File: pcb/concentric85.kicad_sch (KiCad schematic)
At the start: 176 parts, among them J1 USB_C_Receptacle_USB2.0, SW1 SW_Push, SW10 SW_Push, SW11 SW_Push, SW12 SW_Push, SW13 SW_Push, SW14 SW_Push, SW15 SW_Push, SW16 SW_Push, SW17 SW_Push, SW18 SW_Push, SW19 SW_Push, SW2 SW_Push, SW20 SW_Push, SW21 SW_Push, SW22 SW_Push, SW23 SW_Push, SW24 SW_Push, SW25 SW_Push, SW26 SW_Push, SW27 SW_Push, SW28 SW_Push, SW29 SW_Push, SW3 SW_Push, SW30 SW_Push, SW31 SW_Push, SW32 SW_Push, SW33 SW_Push, SW34 SW_Push, SW35 SW_Push, SW36 SW_Push, SW37 SW_Push, SW38 SW_Push, SW39 SW_Push, SW4 SW_Push, SW40 SW_Push, SW41 SW_Push, SW42 SW_Push, SW43 SW_Push, SW44 SW_Push, SW45 SW_Push, SW46 SW_Push, SW47 SW_Push, SW48 SW_Push, SW49 SW_Push, SW5 SW_Push, SW50 SW_Push, SW51 SW_Push, SW52 SW_Push, SW53 SW_Push, SW54 SW_Push, SW55 SW_Push, SW56 SW_Push, SW57 SW_Push, SW58 SW_Push, SW59 SW_Push, SW6 SW_Push, SW60 SW_Push, SW61 SW_Push, SW62 SW_Push, SW63 SW_Push, SW64 SW_Push, SW65 SW_Push, SW66 SW_Push, SW67 SW_Push, SW68 SW_Push, SW69 SW_Push, SW7 SW_Push, SW70 SW_Push, SW71 SW_Push, SW72 SW_Push, SW73 SW_Push, SW74 SW_Push, SW75 SW_Push, SW76 SW_Push, SW77 SW_Push, SW78 SW_Push, SW79 SW_Push, SW8 SW_Push, SW80 SW_Push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

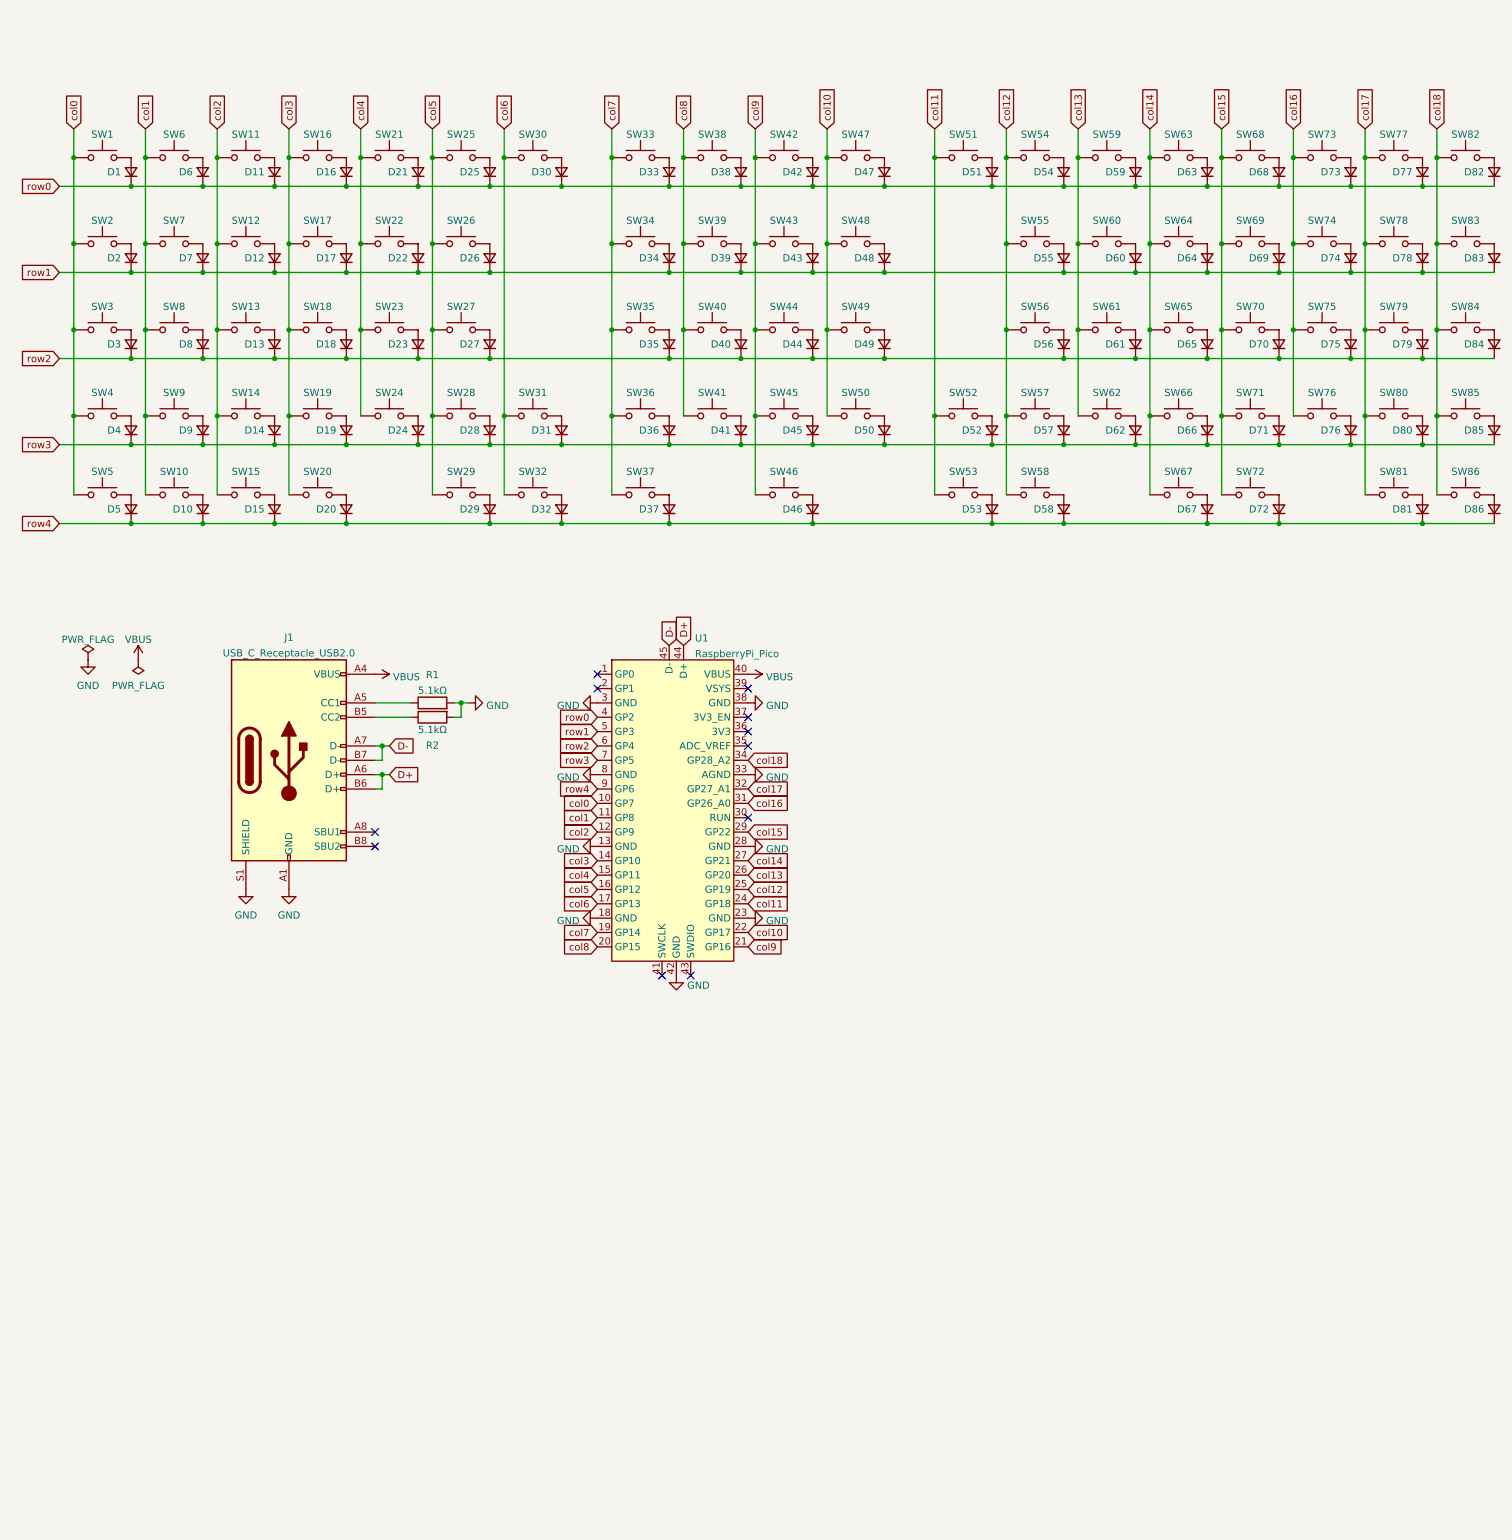
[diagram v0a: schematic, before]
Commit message: backup
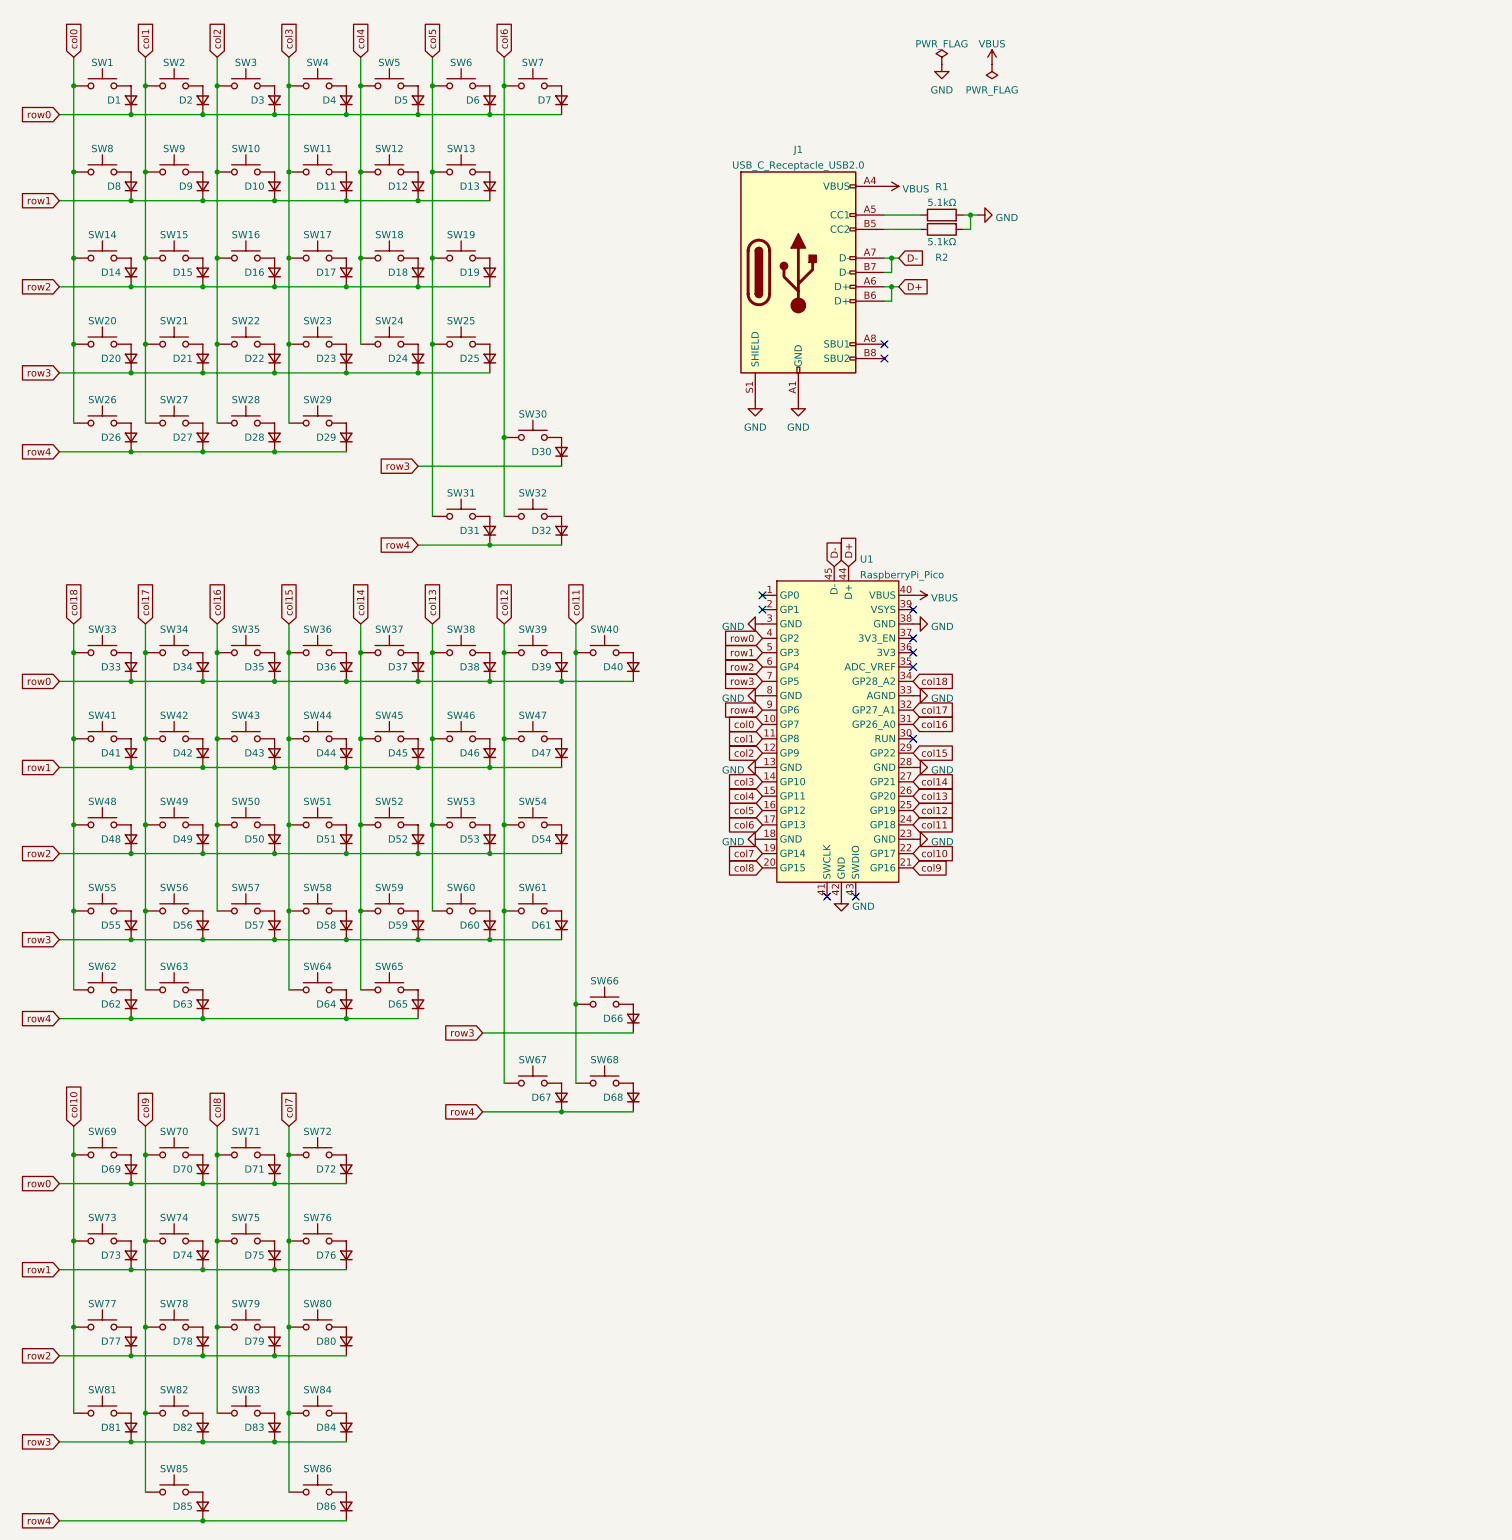
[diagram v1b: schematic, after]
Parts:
- R1, R2: footprint concentric85:MX_1.00u_Hotswap -> Resistor_SMD:R_0805_2012Metric_Pad1.20x1.40mm_HandSolder
- SW63: renamed from SW58; footprint concentric85:MX_1.00u_Hotswap -> concentric85:MX_1.50u_Hotswap
- SW67: renamed from SW81; footprint concentric85:MX_1.50u_Hotswap -> concentric85:MX_1.00u_Hotswap
- SW85: renamed from SW37; footprint concentric85:MX_2.00u_Hotswap -> concentric85:MX_1.00u_Hotswap
- SW86: renamed from SW46; footprint concentric85:MX_1.00u_Hotswap -> concentric85:MX_2.00u_Hotswap
- U1: footprint concentric85:MX_1.50u_Hotswap -> concentric85:RaspberryPi_Pico
- renumbered D12 to D10, D17 to D11, D22 to D12, D26 to D13, D3 to D14, D8 to D15, D13 to D16, D18 to D17, D23 to D18, D27 to D19, D6 to D2, D4 to D20, D9 to D21, D14 to D22, D19 to D23, D28 to D25, D5 to D26, D10 to D27, D15 to D28, D20 to D29, D11 to D3, D31 to D30, D29 to D31, D51 to D33, D54 to D34, D59 to D35, D63 to D36, D68 to D37, D73 to D38, D77 to D39, D16 to D4, D82 to D40, D83 to D41, D55 to D42, D60 to D43, D64 to D44, D69 to D45, D74 to D46, D78 to D47, D84 to D48, D56 to D49, D21 to D5, D61 to D50, D65 to D51, D70 to D52, D75 to D53, D79 to D54, D52 to D55, D57 to D56, D62 to D57, D66 to D58, D71 to D59, D25 to D6, D76 to D60, D80 to D61, D53 to D62, D58 to D63, D67 to D64, D72 to D65, D85 to D66, D81 to D67, D86 to D68, D33 to D69, D30 to D7, D38 to D70, D42 to D71, D47 to D72, D34 to D73, D39 to D74, D43 to D75, D48 to D76, D35 to D77, D40 to D78, D44 to D79, D2 to D8, D49 to D80, D36 to D81, D41 to D82, D45 to D83, D50 to D84, D37 to D85, D46 to D86, D7 to D9, SW12 to SW10, SW17 to SW11, SW22 to SW12, SW26 to SW13, SW3 to SW14, SW8 to SW15, SW13 to SW16, SW18 to SW17, SW23 to SW18, SW27 to SW19, SW6 to SW2, SW4 to SW20, SW9 to SW21, SW14 to SW22, SW19 to SW23, SW28 to SW25, SW5 to SW26, SW10 to SW27, SW15 to SW28, SW20 to SW29, SW11 to SW3, SW31 to SW30, SW29 to SW31, SW51 to SW33, SW54 to SW34, SW59 to SW35, SW63 to SW36, SW68 to SW37, SW73 to SW38, SW77 to SW39, SW16 to SW4, SW82 to SW40, SW83 to SW41, SW55 to SW42, SW60 to SW43, SW64 to SW44, SW69 to SW45, SW74 to SW46, SW78 to SW47, SW84 to SW48, SW56 to SW49, SW21 to SW5, SW61 to SW50, SW65 to SW51, SW70 to SW52, SW75 to SW53, SW79 to SW54, SW52 to SW55, SW57 to SW56, SW62 to SW57, SW66 to SW58, SW71 to SW59, SW25 to SW6, SW76 to SW60, SW80 to SW61, SW53 to SW62, SW67 to SW64, SW72 to SW65, SW85 to SW66, SW86 to SW68, SW33 to SW69, SW30 to SW7, SW38 to SW70, SW42 to SW71, SW47 to SW72, SW34 to SW73, SW39 to SW74, SW43 to SW75, SW48 to SW76, SW35 to SW77, SW40 to SW78, SW44 to SW79, SW2 to SW8, SW49 to SW80, SW36 to SW81, SW41 to SW82, SW45 to SW83, SW50 to SW84, SW7 to SW9
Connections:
- net col10: now also SW69.1, SW73.1, SW77.1, SW81.1; no longer SW72.1, SW76.1, SW80.1, SW84.1
- net col11: now also SW40.1, SW66.1, SW68.1; no longer SW33.1, SW55.1, SW62.1
- net col12: now also SW39.1, SW47.1, SW54.1, SW61.1, SW67.1; no longer SW34.1, SW42.1, SW49.1, SW56.1, SW63.1
- net col13: now also SW38.1, SW46.1, SW53.1, SW60.1; no longer SW35.1, SW43.1, SW50.1, SW57.1
- net col14: now also SW37.1, SW45.1, SW52.1, SW59.1, SW65.1; no longer SW36.1, SW44.1, SW51.1, SW58.1, SW64.1
- net col15: now also SW36.1, SW44.1, SW51.1, SW58.1, SW64.1; no longer SW37.1, SW45.1, SW52.1, SW59.1, SW65.1
- net col16: now also SW35.1, SW43.1, SW50.1, SW57.1; no longer SW38.1, SW46.1, SW53.1, SW60.1
- net col17: now also SW34.1, SW42.1, SW49.1, SW56.1, SW63.1; no longer SW39.1, SW47.1, SW54.1, SW61.1, SW67.1
- net col18: now also SW33.1, SW55.1, SW62.1; no longer SW40.1, SW66.1, SW68.1
- net col7: now also SW72.1, SW76.1, SW80.1, SW84.1, SW86.1; no longer SW69.1, SW73.1, SW77.1, SW81.1, SW85.1
- net col8: now also SW71.1, SW75.1, SW79.1, SW83.1; no longer SW70.1, SW74.1, SW78.1, SW82.1
- net col9: now also SW70.1, SW74.1, SW78.1, SW82.1, SW85.1; no longer SW71.1, SW75.1, SW79.1, SW83.1, SW86.1
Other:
- moved on the sheet: D1, D10, D11, D12, D13, D14, D15, D16, D17, D18, D19, D2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
